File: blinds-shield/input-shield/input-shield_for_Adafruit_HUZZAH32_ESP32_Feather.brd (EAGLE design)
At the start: 50.8 x 22.9 mm, 18 parts

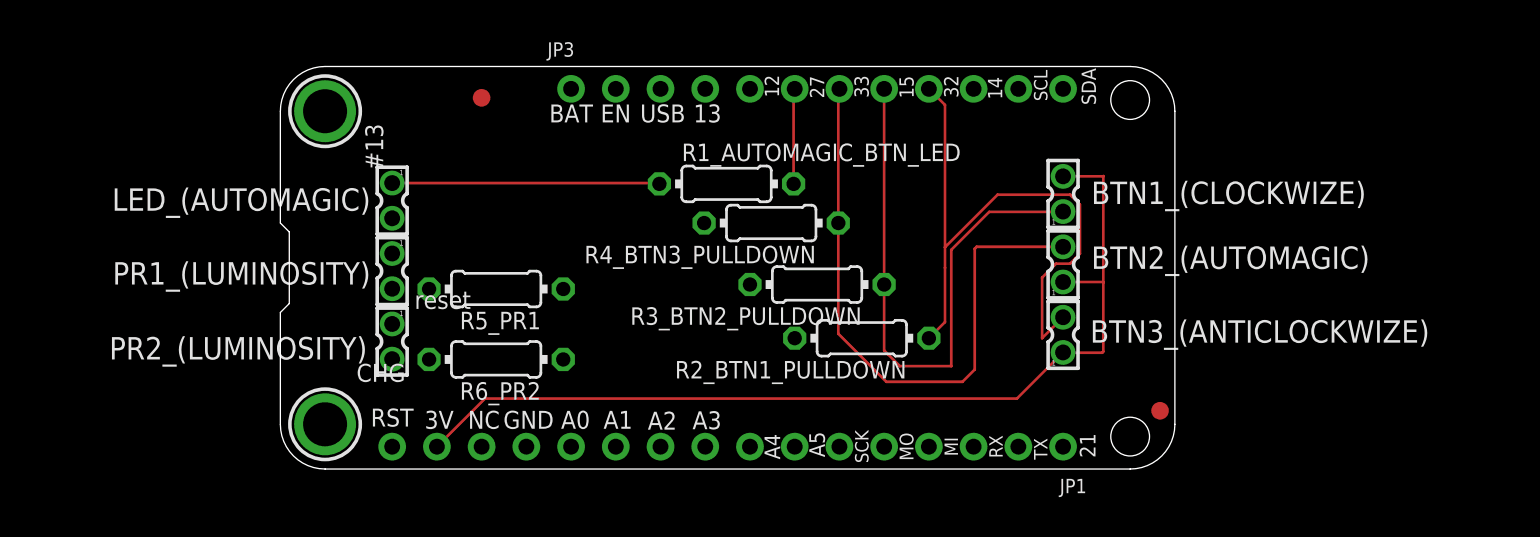
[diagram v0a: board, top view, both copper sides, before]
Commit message: Add files via upload
nu shieeeld
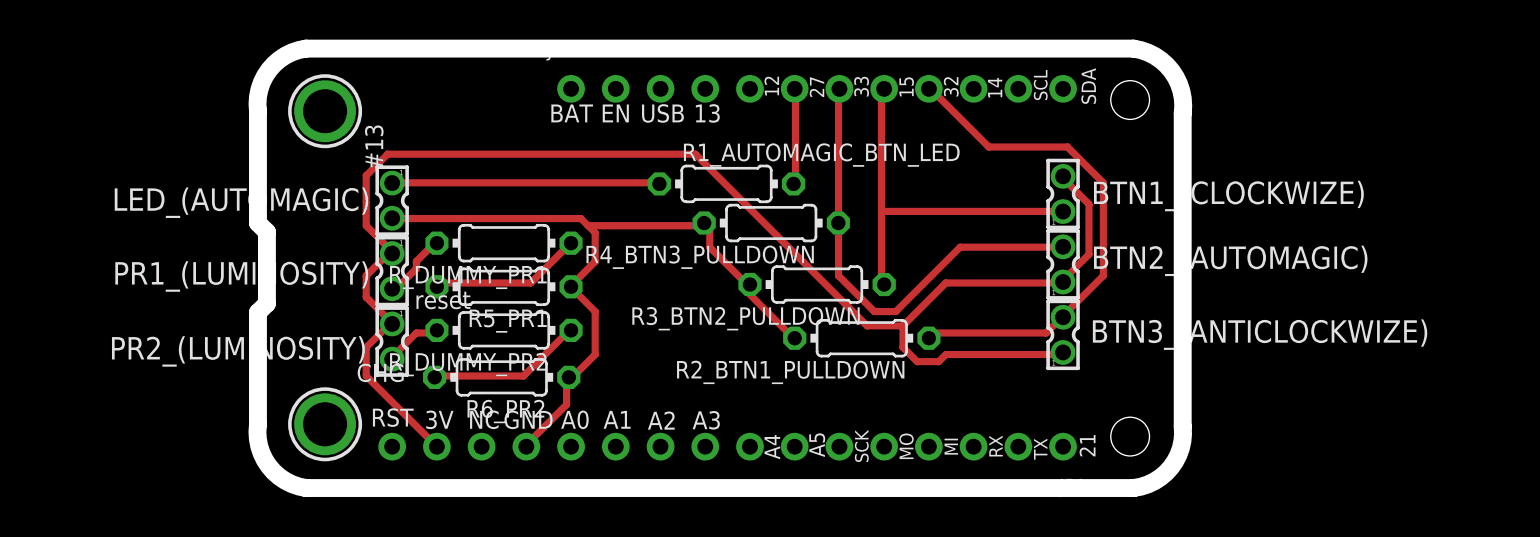
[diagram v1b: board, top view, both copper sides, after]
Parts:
- removed U$34, U$35: FIDUCIAL_1MM, microbuilder:FIDUCIAL_1MM
- added R_DUMMY_PR1, R_DUMMY_PR2: 0k ohm, rcl:0204/7
- moved R6_PR2 1.06 mm to (12.6, 5.21)
- moved R5_PR1 0.46 mm to (12.7, 10.4)
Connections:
- new net N$4: R5_PR1.2, R_DUMMY_PR1.1
- new net N$5: R6_PR2.2, R_DUMMY_PR2.1
- net N$2: now also R_DUMMY_PR1.2; no longer R5_PR1.2
- net N$3: now also R_DUMMY_PR2.2; no longer R6_PR2.2
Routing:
- net GND: track 0.00 -> 42.5 mm
- net 3.3V: track 54.6 -> 82.8 mm
- net IO15_A8: track 32.9 -> 21.6 mm
- net IO33_A9: track 35.0 -> 25.7 mm
- net N$5: track 0.00 -> 8.81 mm
- net N$4: track 0.00 -> 8.72 mm
- net IO32_A7: track 34.7 -> 28.8 mm
- net N$2: track 0.00 -> 3.87 mm
- net N$3: track 0.00 -> 3.23 mm
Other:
- board size 50.8 x 22.9 mm -> 52.6 x 25 mm
